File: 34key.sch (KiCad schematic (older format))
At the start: 22 parts, among them J1 AudioJack4dpb, SW10 SW_Push, SW11 SW_Push, SW12 SW_Push, SW14 SW_Push, SW15 SW_Push, SW16 SW_Push, SW17 SW_Push, SW18 SW_Push, SW2 SW_Push, SW20 SW_Push, SW21 SW_Push, SW3 SW_Push, SW4 SW_Push, SW5 SW_Push, SW6 SW_Push, SW8 SW_Push, SW9 SW_Push, U1 ProMicro-kbd

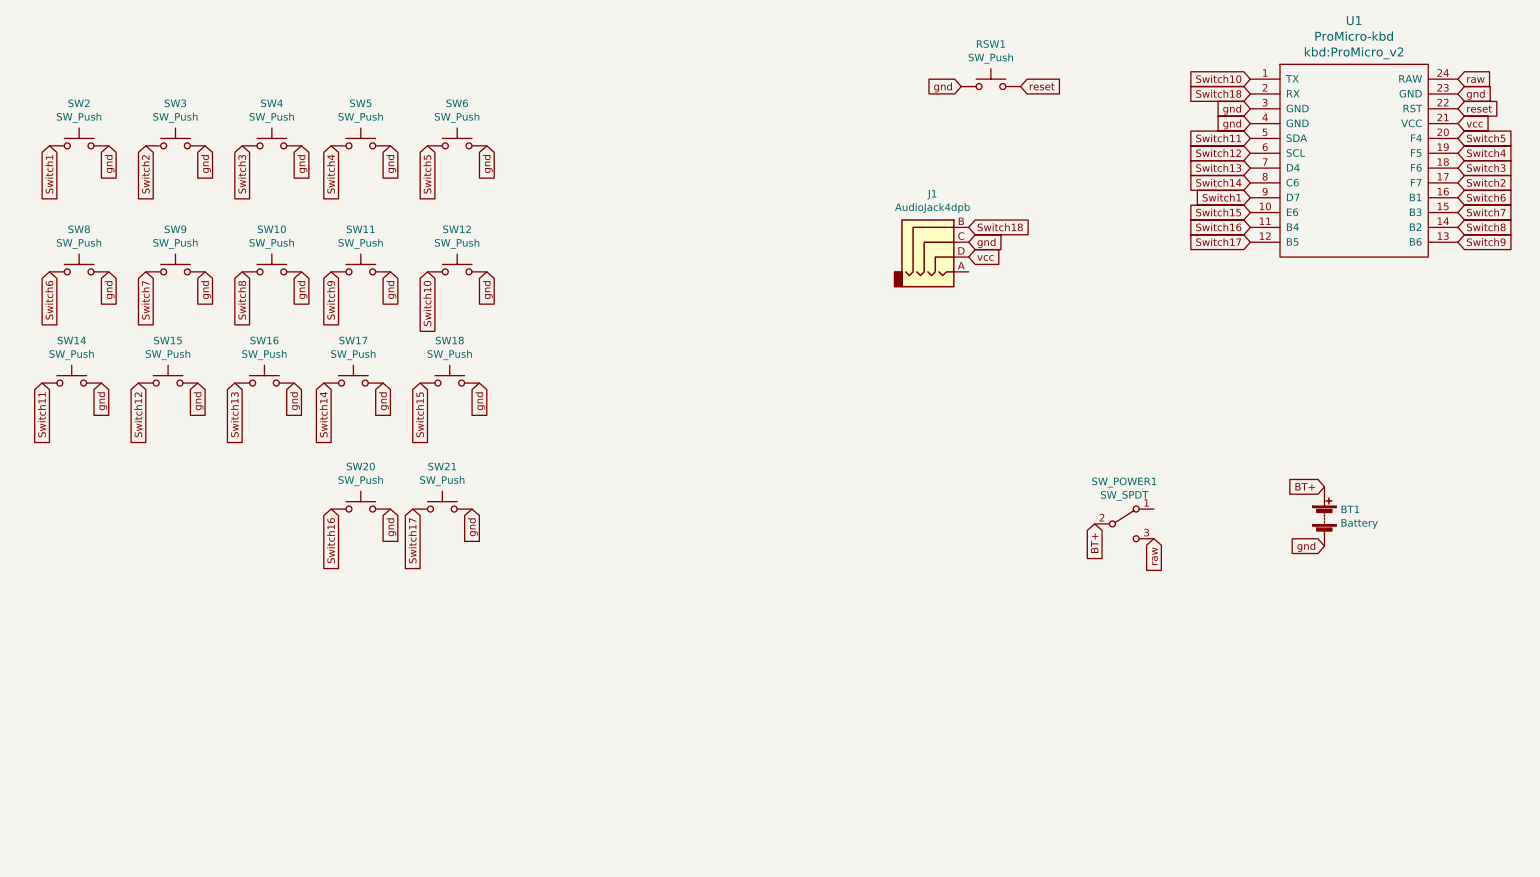
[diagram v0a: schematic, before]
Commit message: Add files via upload
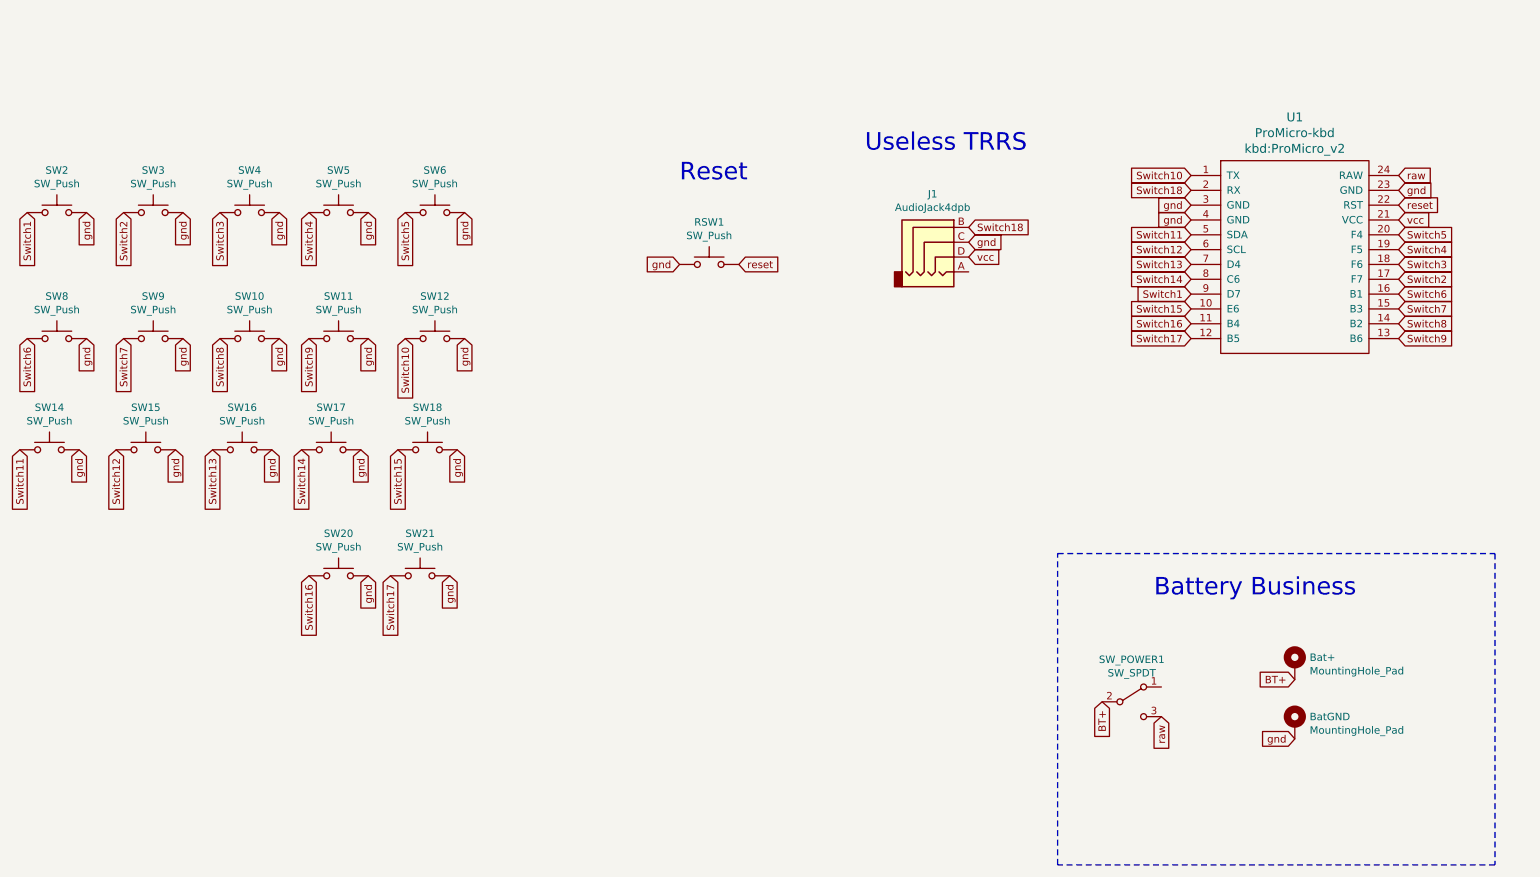
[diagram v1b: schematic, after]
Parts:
- removed BT1: Battery, Battery:BatteryHolder_Keystone_2998_1x6.8mm, symbol Device:Battery
- added Bat+, BatGND: MountingHole_Pad, kbd:1pin_conn, symbol Mechanical:MountingHole_Pad
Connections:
- net BT+: now also Bat+.1
- net gnd: now also BatGND.1
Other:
- note added: "Battery Business"
- note added: "Reset"
- note added: "Useless TRRS\n"
- moved on the sheet: RSW1, SW10, SW11, SW12, SW14, SW15, SW16, SW17, SW18, SW2, SW20, SW21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
